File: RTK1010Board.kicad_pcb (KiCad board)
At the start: 2 copper layers, 56.2 x 53.3 mm, 53 parts, among them J1 SMA, J2 IPEX, J3 USB_OTG, U1 RTK-1010, U2 MCP1700-3002E_SOT23, U3 MCP1700-3002E_SOT23, U4 ESP32-S2-WROVER

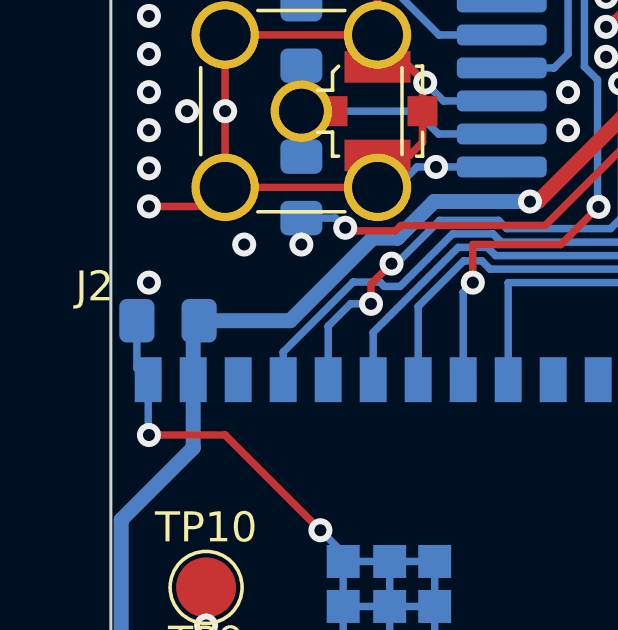
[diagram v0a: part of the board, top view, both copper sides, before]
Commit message: gerber files created
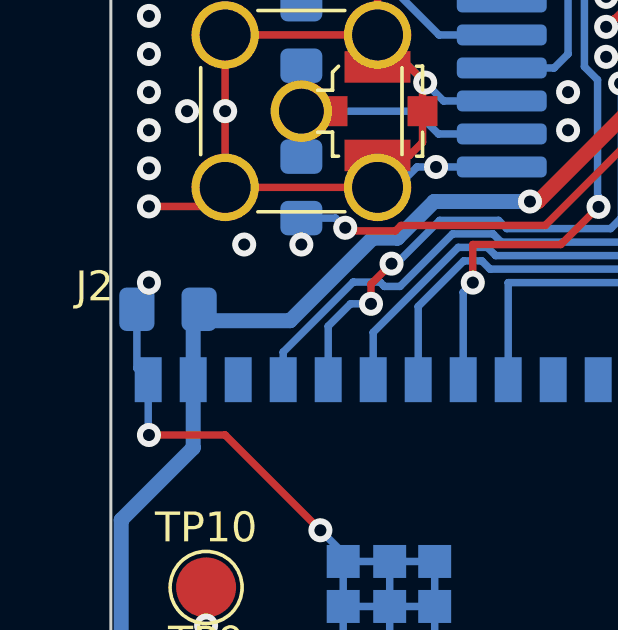
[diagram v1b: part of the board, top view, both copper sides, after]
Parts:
- moved C8 0.38 mm to (173.4, 95.5)
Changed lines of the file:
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@@
       (drillshape 0)
       (scaleselection 1)
-      (outputdirectory "out")
+      (outputdirectory "gerber")
     )
   )
@@
       (net 35 "EN") (pinfunction "D5") (pintype "bidirectional+no_connect"))
     (pad "D6" thru_hole oval (at 35.814 -50.8) (size 1.7272 2.5) (drill 1.016 (offset 0 -0.5)) (layers *.Cu *.Mask)
-      (net 36 "GPIO26") (pinfunction "D6") (pintype "bidirectional+no_connect"))
+      (net 36 "GPIO26") (pinfunction "D6") (pintype "bidirectional"))
     (pad "D7" thru_hole oval (at 33.274 -50.8) (size 1.7272 2.5) (drill 1.016 (offset 0 -0.5)) (layers *.Cu *.Mask)
       (net 37 "LNA_EN") (pinfunction "D7") (pintype "bidirectional"))
@@
       (net 43 "_GPIO26") (pintype "passive"))
     (pad "2" smd roundrect (at 1 0 90) (size 1.2 1.4) (layers "B.Cu" "B.Paste" "B.Mask") (roundrect_rratio 0.2083333333)
-      (net 36 "GPIO26") (pintype "passive+no_connect"))
+      (net 36 "GPIO26") (pintype "passive"))
     (model "${KICAD6_3DMODEL_DIR}/Resistor_SMD.3dshapes/R_0805_2012Metric.wrl"
       (offset (xyz 0 0 0))
@@
   )
   (footprint "Capacitor_SMD:C_0805_2012Metric_Pad1.18x1.45mm_HandSolder" (layer "B.Cu")
-    (at 173.355 95.885 180)
+    (at 173.355 95.504 180)
     (descr "Capacitor SMD 0805 (2012 Metric), square (rectangular) end terminal, IPC_7351 nominal with elongated pad for handsoldering. (Body size source: IPC-SM-782 page 76, https://www.pcb-3d.com/wordpress/wp-content/uploads/ipc-sm-782a_amendment_1_and_2.pdf, https://docs.google.com/spreadsheets/d/1BsfQQcO9C6DZCsRaXUlFlo91Tg2WpOkGARC1WS5S8t0/edit?usp=sharing), generated with kicad-footprint-generator")
     (tags "capacitor handsolder")
